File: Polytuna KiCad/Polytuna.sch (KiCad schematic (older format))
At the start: 45 parts, among them IC1 AP7313-33SAG-7, J1 Barrel_Jack, J2 Conn_01x02, J3 Conn_01x02, J4 Conn_01x04, J5 Conn_01x02, SW1 SW_Push, SW2 SW_Push, SW3 SW_Push, SW4 SW_TPDT, U1 LM358, U2 SGTL5000, U3 L7805

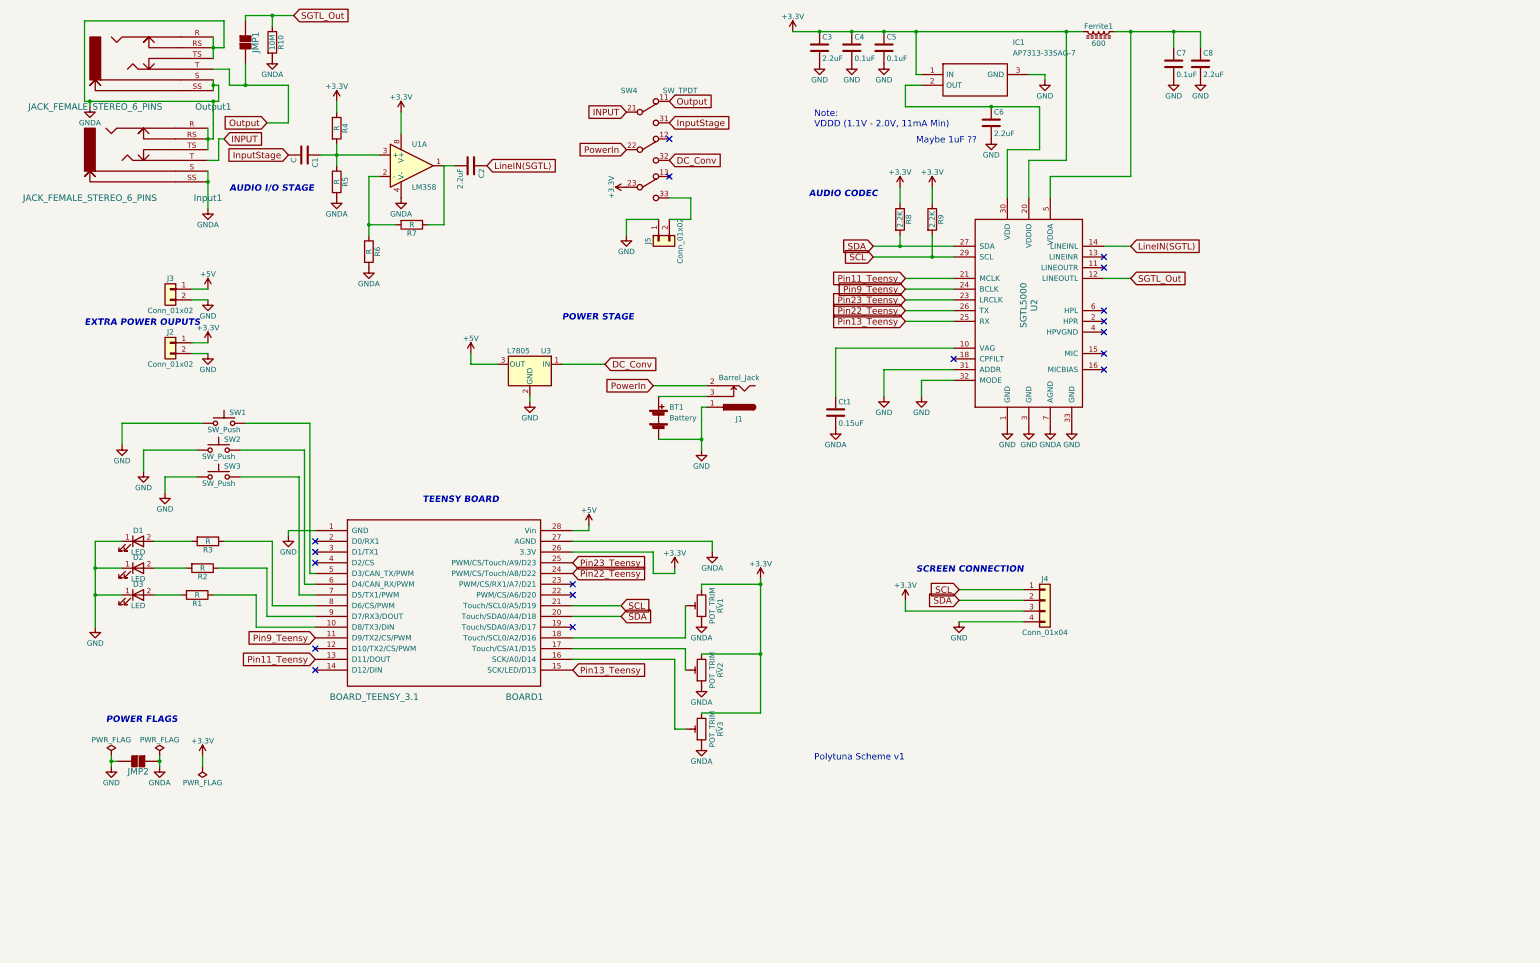
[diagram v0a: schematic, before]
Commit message: Some fixes
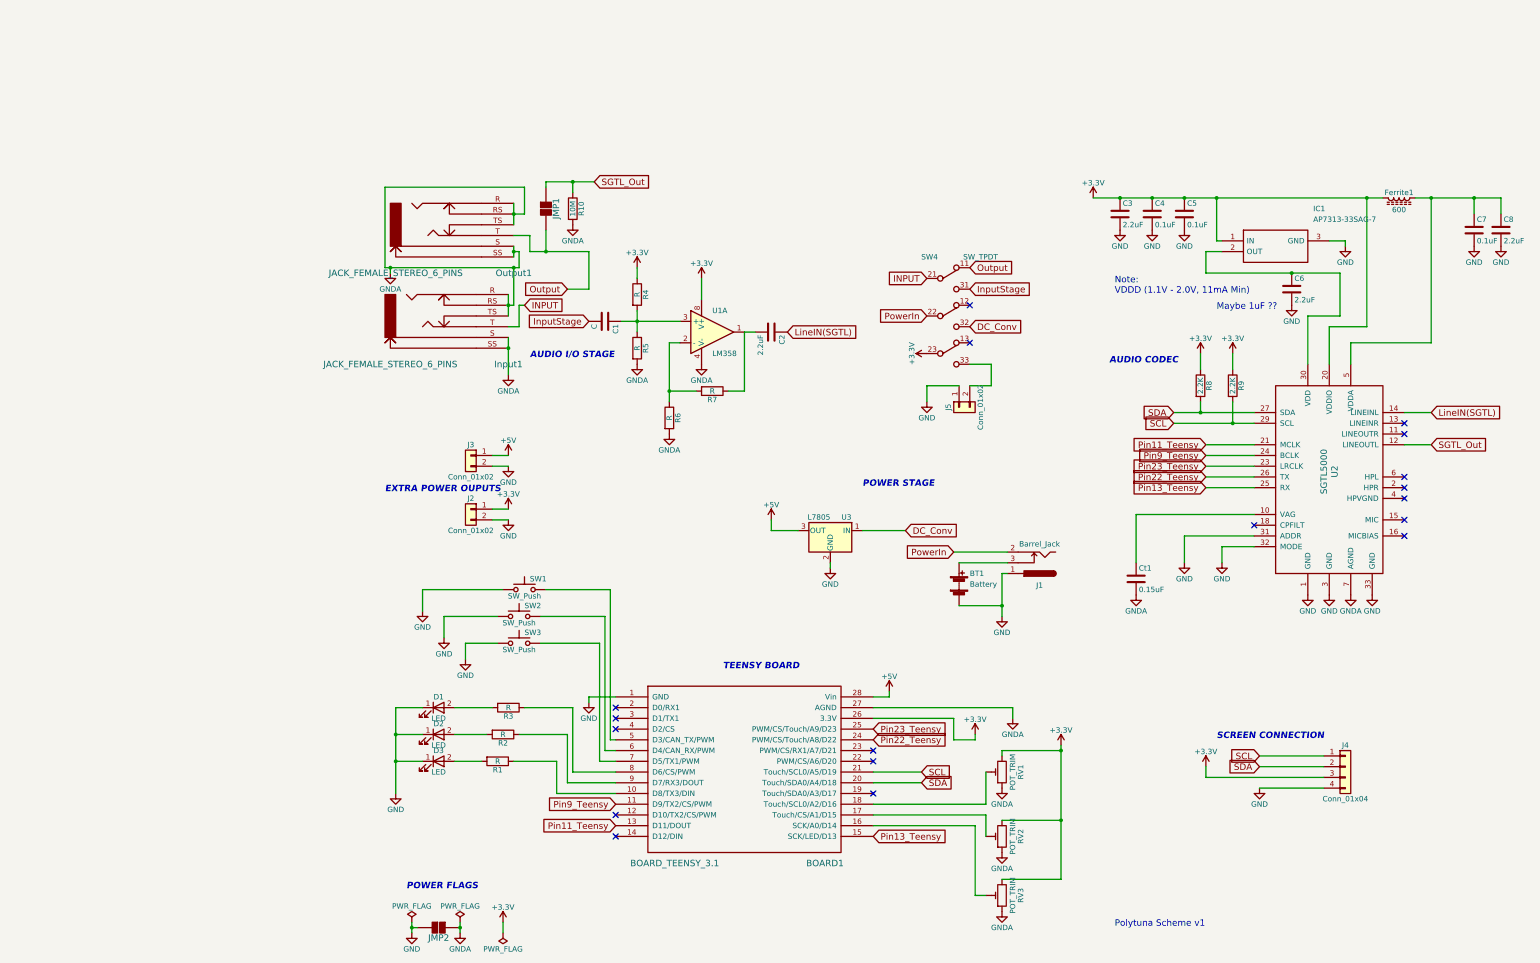
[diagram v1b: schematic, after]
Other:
- moved on the sheet: BOARD1, BT1, C1, C2, C3, C4, C5, C6, C7, C8, Ct1, D1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
